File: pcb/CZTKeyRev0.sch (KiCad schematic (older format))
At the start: 166 parts, among them U1 proton_c

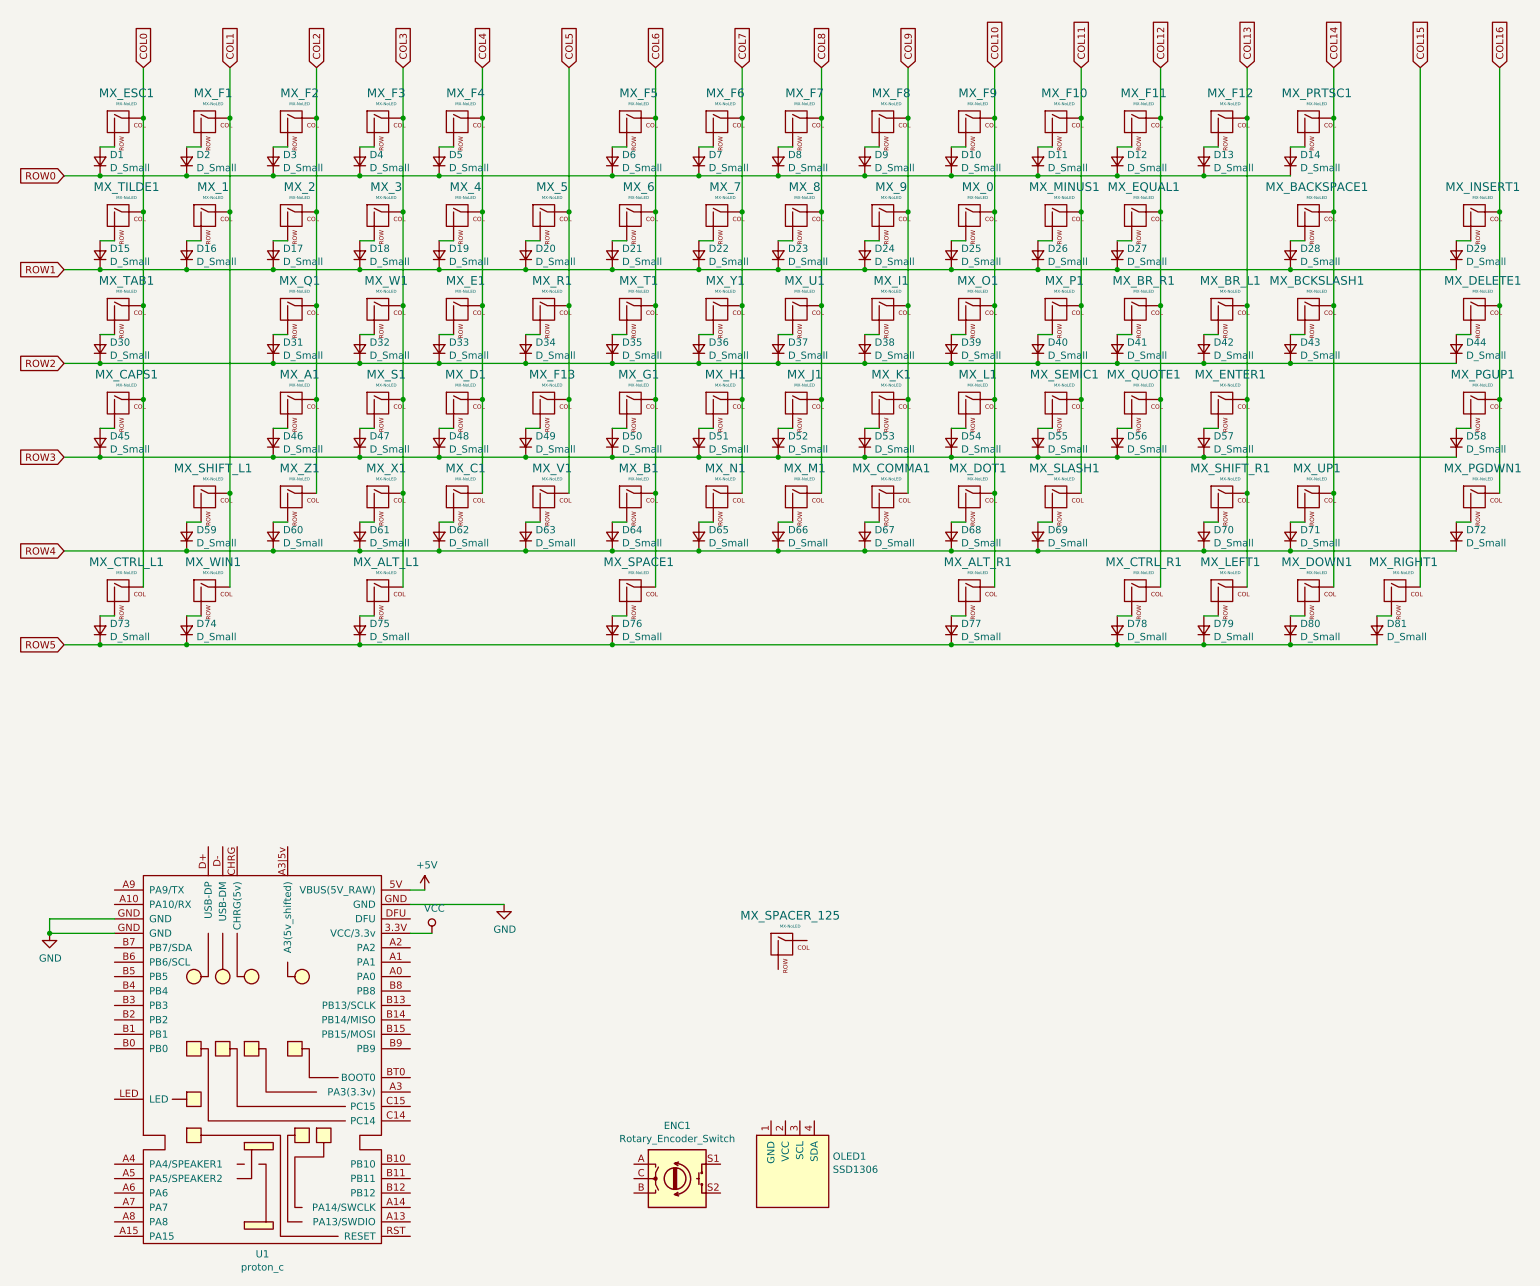
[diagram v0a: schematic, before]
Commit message: Edits to layout and sutff
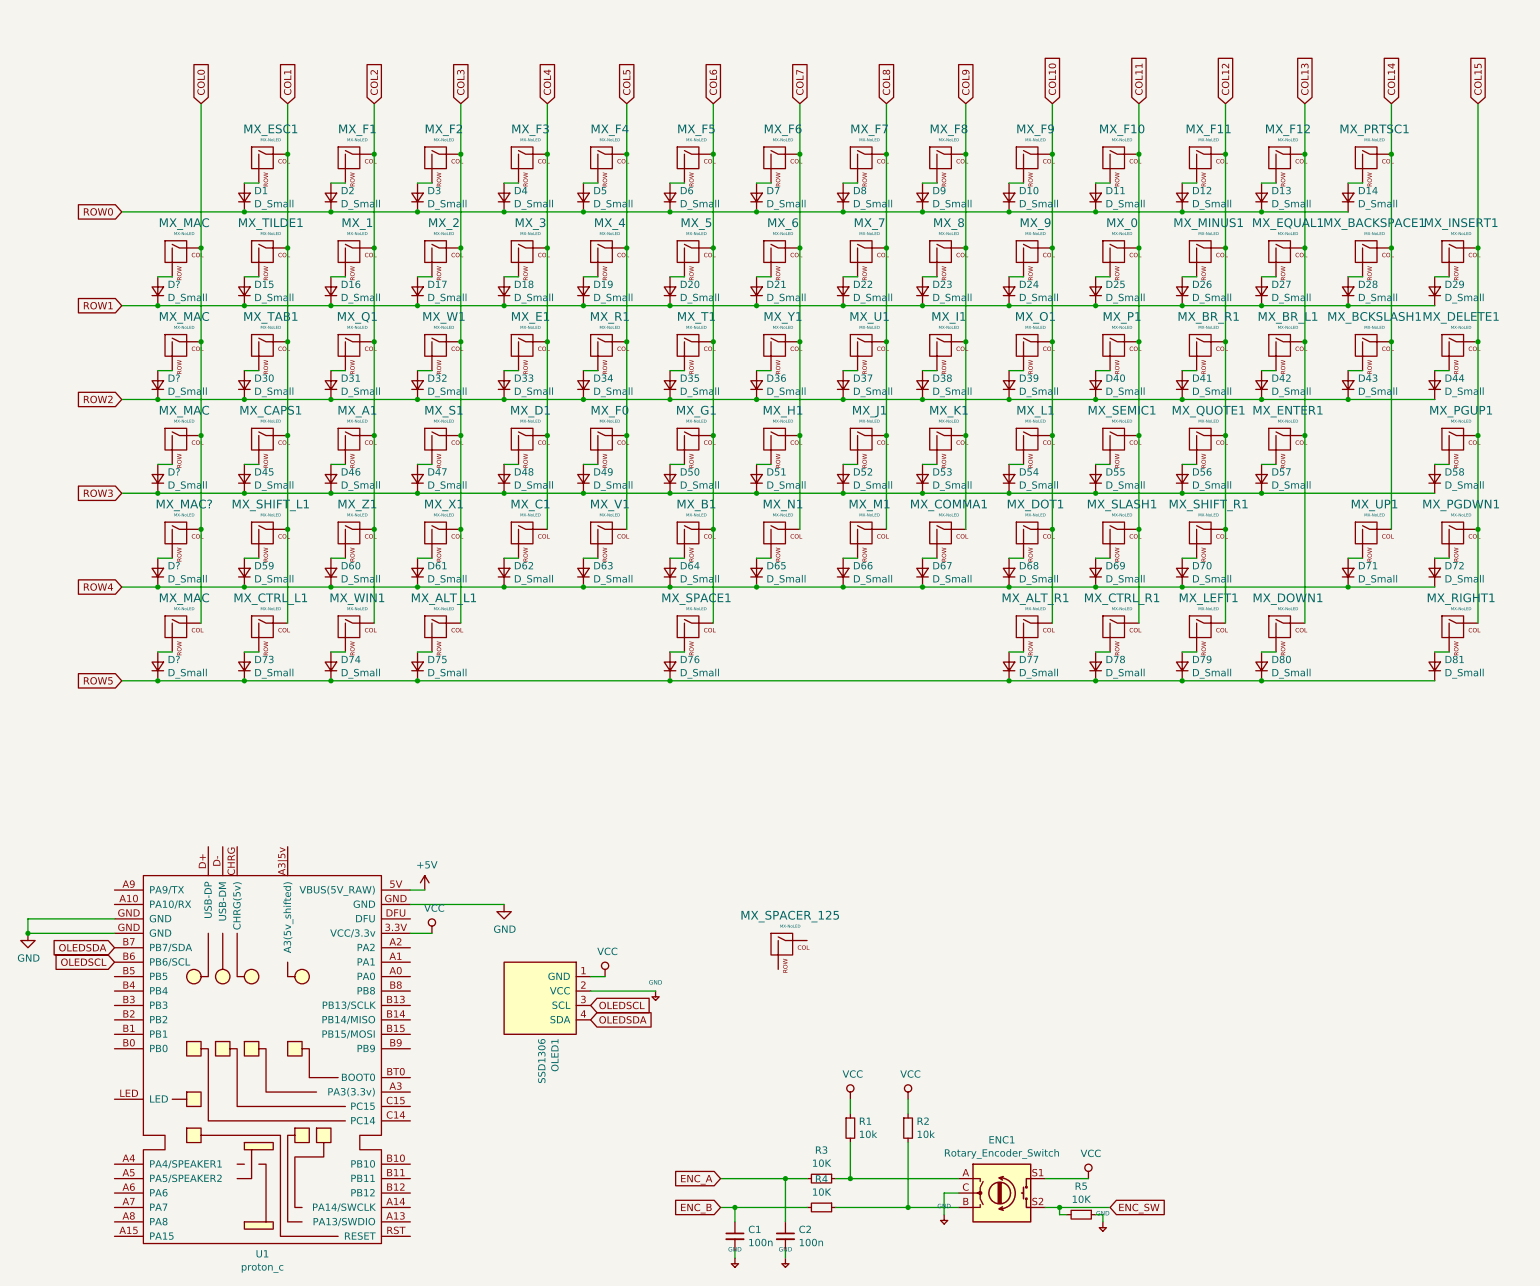
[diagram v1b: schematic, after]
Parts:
- added C1, C2: 100n, symbol Device:C_Small
- added D? (x5): D_Small, Diode_THT:D_DO-35_SOD27_P5.08mm_Vertical_KathodeUp, symbol Device:D_Small
- added MX_MAC: MX-NoLED, MX_Alps_Hybrid:MX-1.25U-NoLED, symbol MX_Alps_Hybrid:MX-NoLED
- added MX_MAC, MX_MAC?: MX-NoLED, MX_Alps_Hybrid:MX-1.75U-NoLED, symbol MX_Alps_Hybrid:MX-NoLED
- added MX_MAC: MX-NoLED, MX_Alps_Hybrid:MX-1.5U-NoLED, symbol MX_Alps_Hybrid:MX-NoLED
- added MX_MAC: MX-NoLED, MX_Alps_Hybrid:MX-1U-NoLED, symbol MX_Alps_Hybrid:MX-NoLED
- added R1, R2: 10k, symbol Device:R_Small
- added R3, R4, R5: 10K, symbol Device:R_Small
- renumbered MX_F13 to MX_F0
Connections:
- net COL16 is gone; now on net COL15: MX_DELETE1.1 (COL), MX_INSERT1.1 (COL), MX_PGDWN1.1 (COL), MX_PGUP1.1 (COL)
- net +5V: now also ENC1.C, OLED1.2 (VCC), C1.2, C2.2, R5.1
- net COL0: now also MX_MAC.1 (COL), MX_MAC.1 (COL), MX_MAC.1 (COL), MX_MAC.1 (COL), MX_MAC?.1 (COL); no longer MX_CAPS1.1 (COL), MX_CTRL_L1.1 (COL), MX_ESC1.1 (COL), MX_TAB1.1 (COL), MX_TILDE1.1 (COL)
- net COL1: now also MX_CAPS1.1 (COL), MX_CTRL_L1.1 (COL), MX_ESC1.1 (COL), MX_TAB1.1 (COL), MX_TILDE1.1 (COL); no longer MX_1.1 (COL), MX_F1.1 (COL), MX_WIN1.1 (COL)
- net COL10: now also MX_9.1 (COL); no longer MX_0.1 (COL)
- net COL11: now also MX_0.1 (COL), MX_CTRL_R1.1 (COL); no longer MX_MINUS1.1 (COL)
- net COL12: now also MX_LEFT1.1 (COL), MX_MINUS1.1 (COL), MX_SHIFT_R1.1 (COL); no longer MX_CTRL_R1.1 (COL), MX_EQUAL1.1 (COL)
- net COL13: now also MX_DOWN1.1 (COL), MX_EQUAL1.1 (COL); no longer MX_LEFT1.1 (COL), MX_SHIFT_R1.1 (COL)
- net COL14: no longer MX_DOWN1.1 (COL)
- net COL2: now also MX_1.1 (COL), MX_F1.1 (COL), MX_WIN1.1 (COL); no longer MX_2.1 (COL), MX_F2.1 (COL)
- net COL3: now also MX_2.1 (COL), MX_F2.1 (COL); no longer MX_3.1 (COL), MX_F3.1 (COL)
- net COL4: now also MX_3.1 (COL), MX_F3.1 (COL); no longer MX_4.1 (COL), MX_F4.1 (COL)
- net COL5: now also MX_4.1 (COL), MX_F4.1 (COL); no longer MX_5.1 (COL)
- net COL6: now also MX_5.1 (COL); no longer MX_6.1 (COL)
- net COL7: now also MX_6.1 (COL); no longer MX_7.1 (COL)
- net COL8: now also MX_7.1 (COL); no longer MX_8.1 (COL)
- net COL9: now also MX_8.1 (COL); no longer MX_9.1 (COL)
- net ROW1: now also D?.1 (K)
- net ROW2: now also D?.1 (K)
- net ROW3: now also D?.1 (K)
- net ROW4: now also D?.1 (K)
- net ROW5: now also D?.1 (K)
- net VCC: now also ENC1.S1, OLED1.1 (GND), R1.1, R2.1
- net OLEDSCL: now reaches U1.B6 (PB6/SCL)
- net OLEDSCL: now also OLED1.3 (SCL)
- net OLEDSDA: now reaches U1.B7 (PB7/SDA)
- net OLEDSDA: now also OLED1.4 (SDA)
- net at ENC1.A: now also R1.2, R3.1
- net at ENC1.B: now also R2.2, R4.1
- net ENC_SW: now reaches ENC1.S2
- net ENC_SW: now also R5.2
- new net: D?.2 (A), MX_MAC.2 (ROW) (x4)
- new net: D?.2 (A), MX_MAC?.2 (ROW)
- new net ENC_A: C2.1, R3.2
- new net ENC_B: C1.1, R4.2
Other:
- moved on the sheet: D1, D10, D11, D12, D13, D14, D15, D16, D17, D18, D19, D2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
